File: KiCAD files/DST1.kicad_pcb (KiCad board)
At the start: 2 copper layers, 50 x 100 mm, 61 parts, among them J3 Barrel_Jack_MountingPin, J4 SN49B14B, J5 SN49B14B, Q1 2N3904, Q2 2N3904, Q3 2N3904, U1 TL072

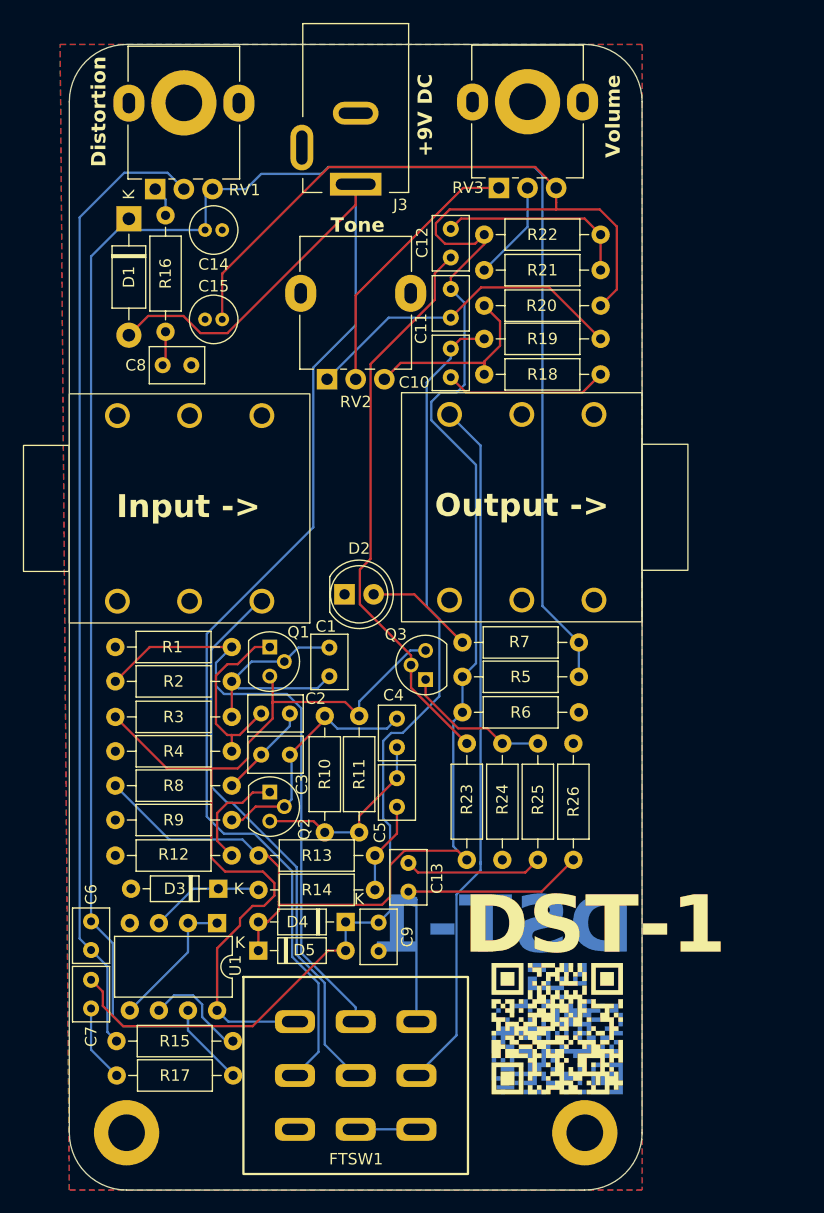
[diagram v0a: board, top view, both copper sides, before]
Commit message: Updated the PCB
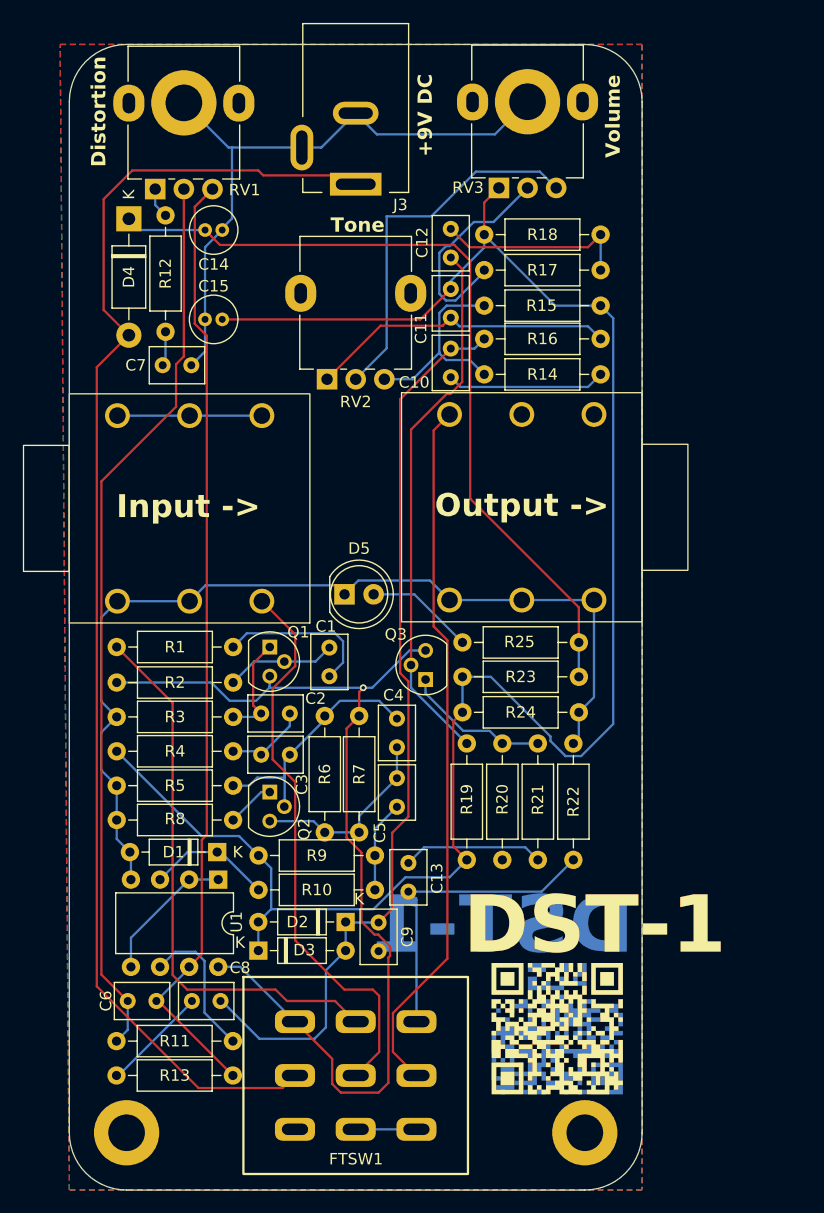
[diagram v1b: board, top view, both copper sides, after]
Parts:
- removed the R1 at (141.7, 92.1)
- C1: value 470nF -> 47nF
- C10: value 100pF -> 22nF
- C11, C9: value 100pF -> 10nF
- R15: renamed from R20; value 2.2kΩ -> 6.8kΩ
- RV3: value 20kΩ -> 100kΩ
- moved C8 8.82 mm to (138.2, 123.0), turned to 0 degrees
- moved C6 5.48 mm to (132.6, 123.0), turned to 0 degrees
- moved U1 3.80 mm to (140.5, 112.4)
- moved D1 3.20 mm to (140.4, 110.0)
- moved R8 3.10 mm to (131.6, 107.2)
- moved R1 3.00 mm to (131.6, 92.1)
- moved R2 3.00 mm to (131.6, 95.2)
- moved R3 3.00 mm to (131.6, 98.2)
- moved R4 3.00 mm to (131.6, 101.2)
- moved R5 3.00 mm to (131.6, 104.2)
- renumbered C8 to C7, C7 to C8, D3 to D1, D4 to D2, D5 to D3, D1 to D4, D2 to D5, R2 to R1, R14 to R10, R15 to R11, R16 to R12, R17 to R13, R18 to R14, R19 to R16, R21 to R17, R22 to R18, R23 to R19, R3 to R2, R24 to R20, R25 to R21, R26 to R22, R5 to R23, R6 to R24, R7 to R25, R4 to R3, R8 to R4, R9 to R5, R10 to R6, R11 to R7, R12 to R8, R13 to R9
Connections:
- C14 pad 1: Net-(C6-Pad2) -> Net-(D4-K)
- D4 pad 1: Net-(C6-Pad2) -> Net-(D4-K)
- R23 pad 2: Net-(C6-Pad2) -> Net-(D4-K)
- R25 pad 2: Net-(C6-Pad2) -> Net-(D4-K)
- RV3 pad 1: Net-(RV2-Pad2) -> +4.5V
- RV3 pad 3: +4.5V -> Net-(RV2-Pad2)
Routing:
- net GND: track 0.00 -> 151.9 mm
- net Net-(C6-Pad2): track 173.3 -> 83.1 mm
- net Net-(D4-K): track 0.00 -> 71.6 mm
- net +4.5V: track 177.5 -> 159.8 mm
- net +9V: track 74.5 -> 89.4 mm, vias 0 -> 1
- net Net-(D2-K): track 90.7 -> 80.3 mm
- net Net-(R17-Pad1): track 8.74 -> 19.0 mm
- net Net-(RV2-Pad2): track 23.7 -> 32.3 mm
- net Net-(Q1-E): track 16.6 -> 9.26 mm
- net Net-(C6-Pad1): track 84.5 -> 78.7 mm
- net Net-(Q2-E): track 9.59 -> 4.21 mm
- net Net-(C1-Pad1): track 9.20 -> 13.9 mm
- net DST_IN: track 52.9 -> 48.3 mm
- net Net-(Q3-B): track 50.8 -> 46.9 mm
- net Net-(U1B--): track 9.31 -> 12.8 mm
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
